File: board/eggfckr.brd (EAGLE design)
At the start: 91.1 x 30.5 mm, 8 parts, among them U1 ATTINY85-20PU

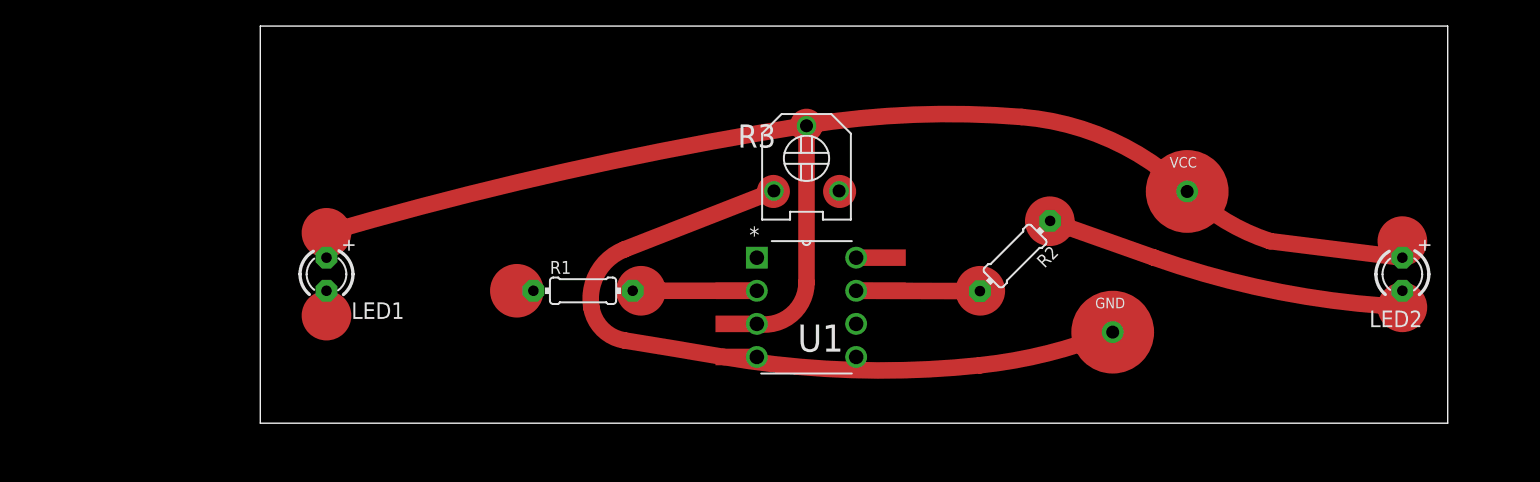
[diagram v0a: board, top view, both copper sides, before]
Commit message: changed routing
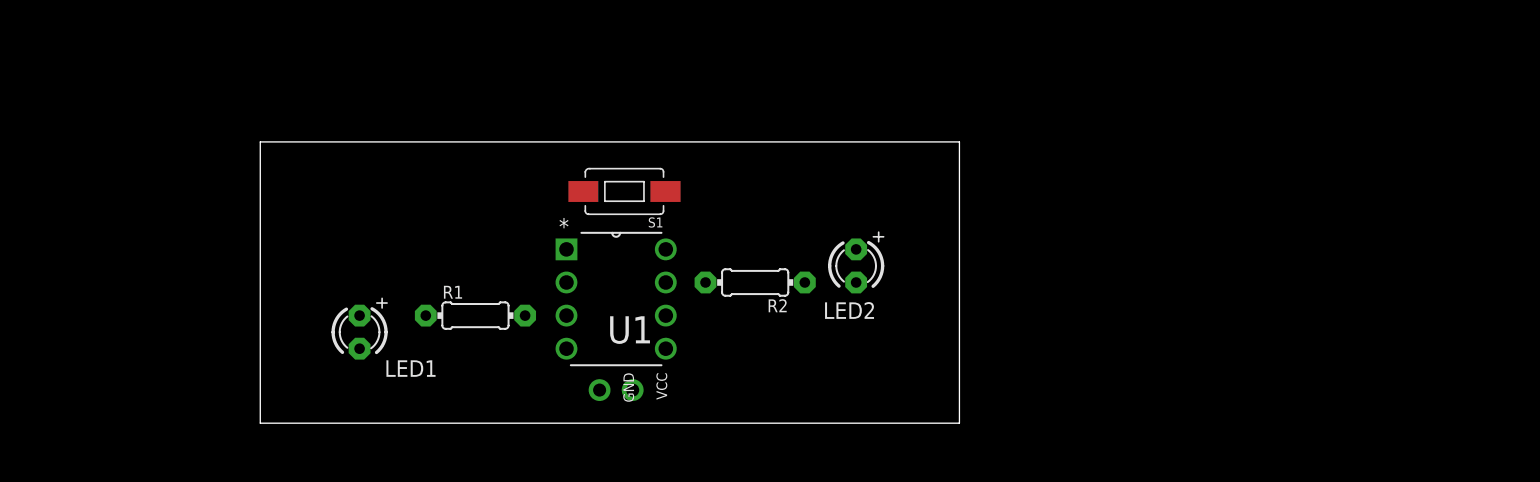
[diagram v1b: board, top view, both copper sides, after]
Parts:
- removed R3: (no value), dp_devices:TRIMMER_3306F
- added S1: SWITCH-MOMENTARY-2-SMD-1101NE, ATtami:TACTILE-SWITCH-1101NE
- moved VCC 45.2 mm to (28.6, 2.54), turned to 270 degrees
- moved LED2 41.9 mm to (45.7, 12.1)
- moved GND 39.6 mm to (26.0, 2.54), turned to 270 degrees
- moved R2 20.0 mm to (38.0, 10.8), turned to 180 degrees
- moved U1 14.6 mm to (31.1, 5.71)
- moved R1 8.47 mm to (16.5, 8.26)
- moved LED1 5.12 mm to (7.62, 6.99)
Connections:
- new net N$5: S1.P$1, U1.2
- net GND: now also LED1.K; no longer R3.1
- net N$2: now also R1.2; no longer R3.2
- net N$3: now also LED1.A; no longer LED1.K
- net N$4: now also S1.P$2, U1.1; no longer R1.2, U1.2
- net VCC: no longer LED1.A, R3.3
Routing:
- net VCC: track 86.5 -> 0.00 mm
- net GND: track 58.9 -> 0.00 mm
- net N$7: track 30.4 -> 0.00 mm
- net N$2: track 17.0 -> 0.00 mm
- net N$4: track 9.53 -> 0.00 mm
- net N$1: track 9.50 -> 0.00 mm
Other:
- board size 91.1 x 30.5 mm -> 53.6 x 21.6 mm

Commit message: dual
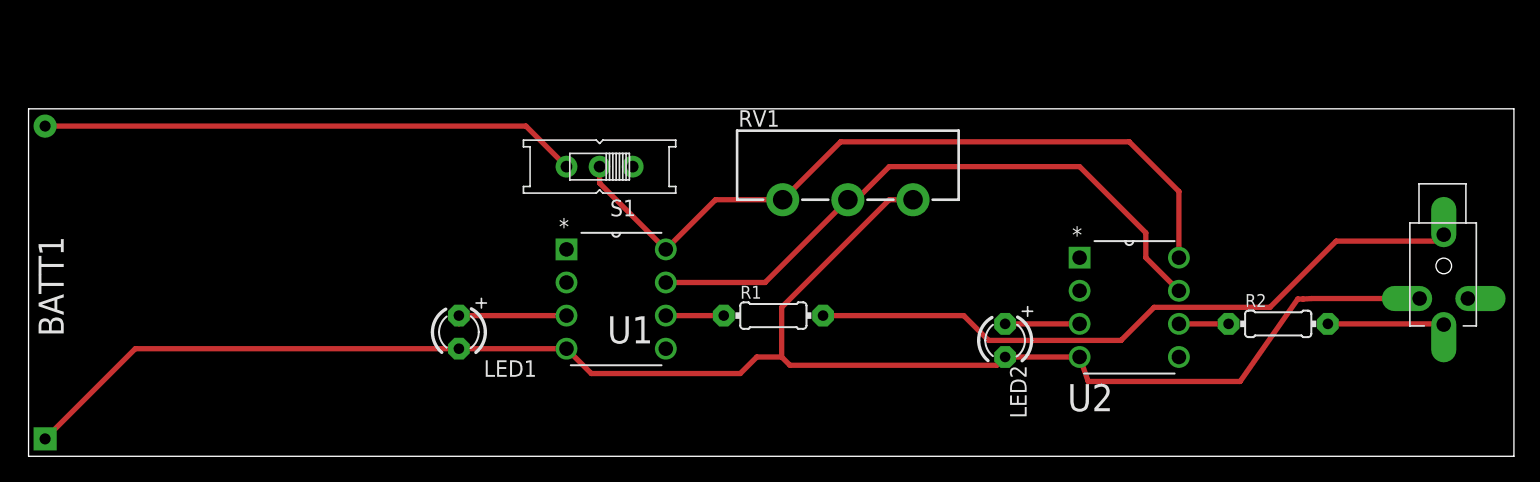
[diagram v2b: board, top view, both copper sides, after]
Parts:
- removed GND, VCC: (no value), microbuilder:1X01_ROUND
- added BATT1: FKIT-COIN_CELLLIR2450-H, SparkFun-Electromechanical:FKIT-LIR2450-H
- added JP1: (no value), SparkFun-Connectors:STEREOJACK2.5MM_SPECIA_POGOPINS
- added RV1: (no value), SparkFun-Electromechanical:POT_ALPHA_RV16AF-20
- added U2: ATTINY85-20PU, Atmel_By_element14_Batch_1-00:DIP254P762X533-8
- S1: value SWITCH-MOMENTARY-2-SMD-1101NE -> (none); device ATtami:TACTILE-SWITCH-1101NE -> adafruit:EG1218
- moved R2 40.3 mm to (78.1, 7.62), turned to 0 degrees
- moved R1 22.9 mm to (39.4, 8.26)
- moved LED2 12.8 mm to (57.1, 6.35)
- moved LED1 7.62 mm to (15.2, 6.99)
- moved S1 2.69 mm to (26.0, 19.7)
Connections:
- new net N$6: LED2.A, U2.3
- new net N$8: BATT1.NEG, S1.S
- net GND: now also BATT1.POS, JP1.RING1, LED2.K, RV1.3, U2.4; no longer GND.1
- net N$1: now also R1.1, U1.6; no longer R2.2, U1.7
- net N$2: now also LED1.A; no longer R1.2
- net N$3: now also JP1.SHIELD, R1.2; no longer LED1.A, R1.1
- net N$4: now also RV1.2, U1.7, U2.7; no longer S1.P$2, U1.1
- net N$5: now also R2.1, U2.6; no longer S1.P$1, U1.2
- net N$7: now also JP1.TIP, R2.2; no longer LED2.K, R2.1
- net VCC: now also RV1.1, S1.P, U2.8; no longer LED2.A, VCC.1
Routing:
- net GND: track 0.00 -> 132.1 mm
- net VCC: track 0.00 -> 57.9 mm
- net N$3: track 0.00 -> 51.8 mm
- net N$4: track 0.00 -> 48.1 mm
- net N$8: track 0.00 -> 41.3 mm
- net N$2: track 0.00 -> 9.15 mm
- net N$7: track 0.00 -> 8.91 mm
- net N$6: track 0.00 -> 5.72 mm
- net N$1: track 0.00 -> 4.45 mm
- net N$5: track 0.00 -> 3.81 mm
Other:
- board size 53.6 x 21.6 mm -> 114 x 26.7 mm
